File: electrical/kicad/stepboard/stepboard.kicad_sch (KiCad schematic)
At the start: 72 parts, among them J1 Conn_02x03_Odd_Even, J10 Conn_01x04, J4 Conn_01x04, J7 Conn_02x03_Odd_Even, U1 TMC2209, U4 TMC2209

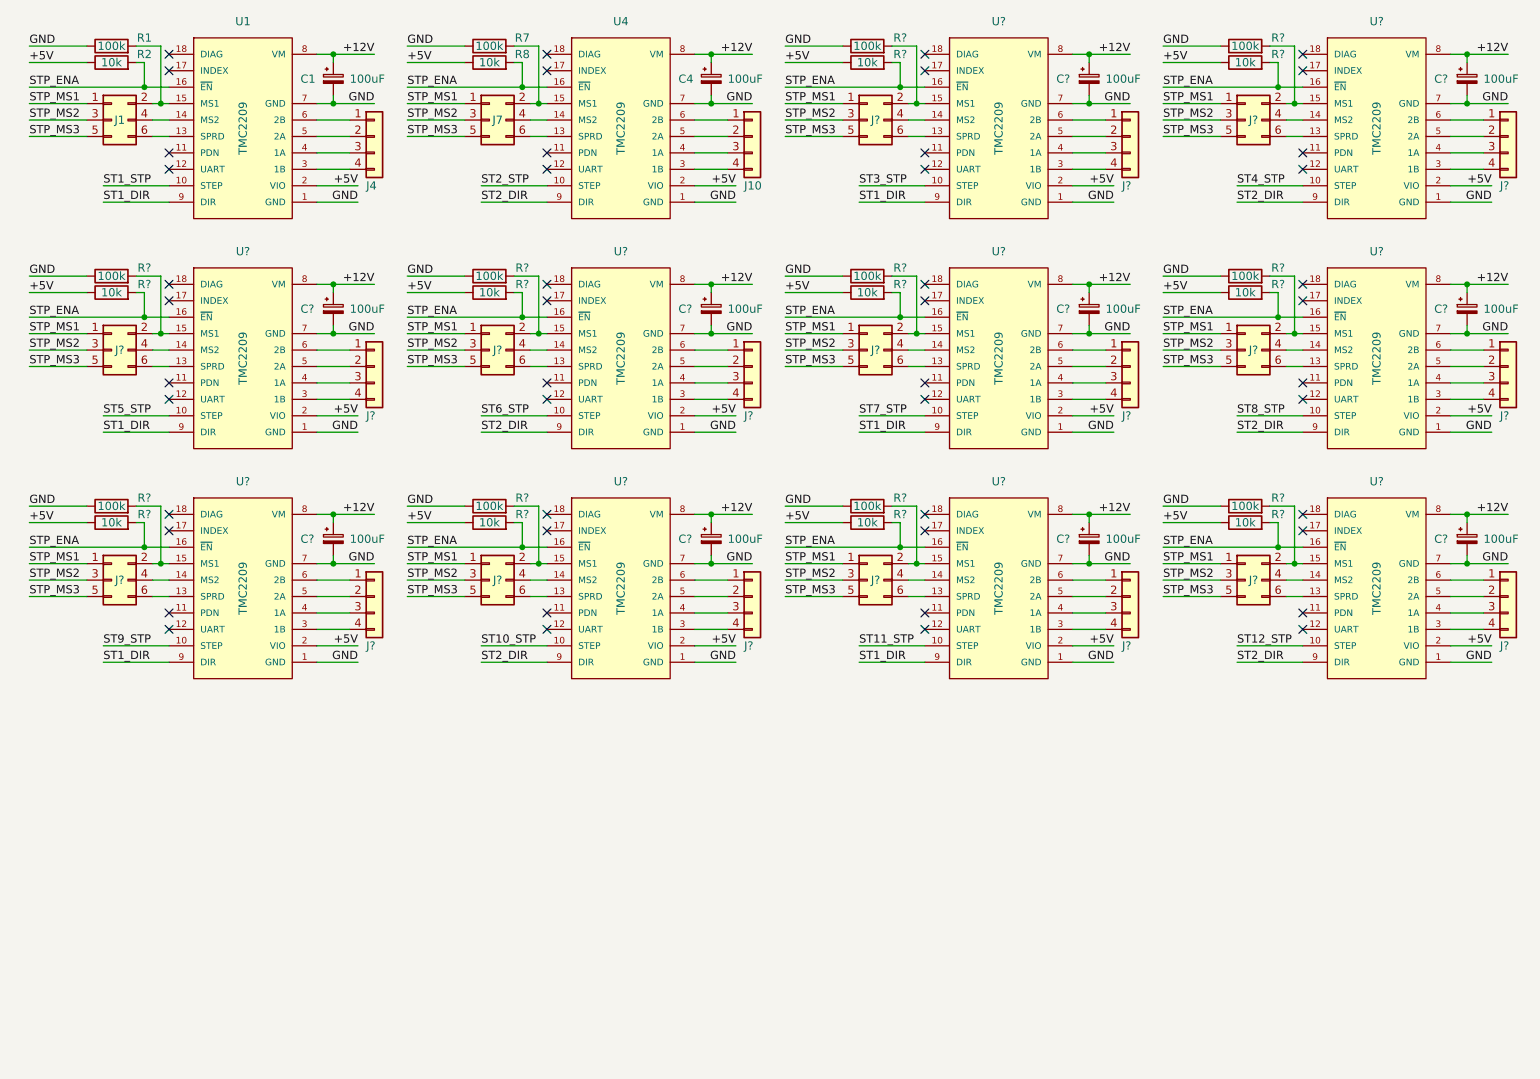
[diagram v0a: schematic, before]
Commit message: update(kicad/step): ERC & DRC Passed
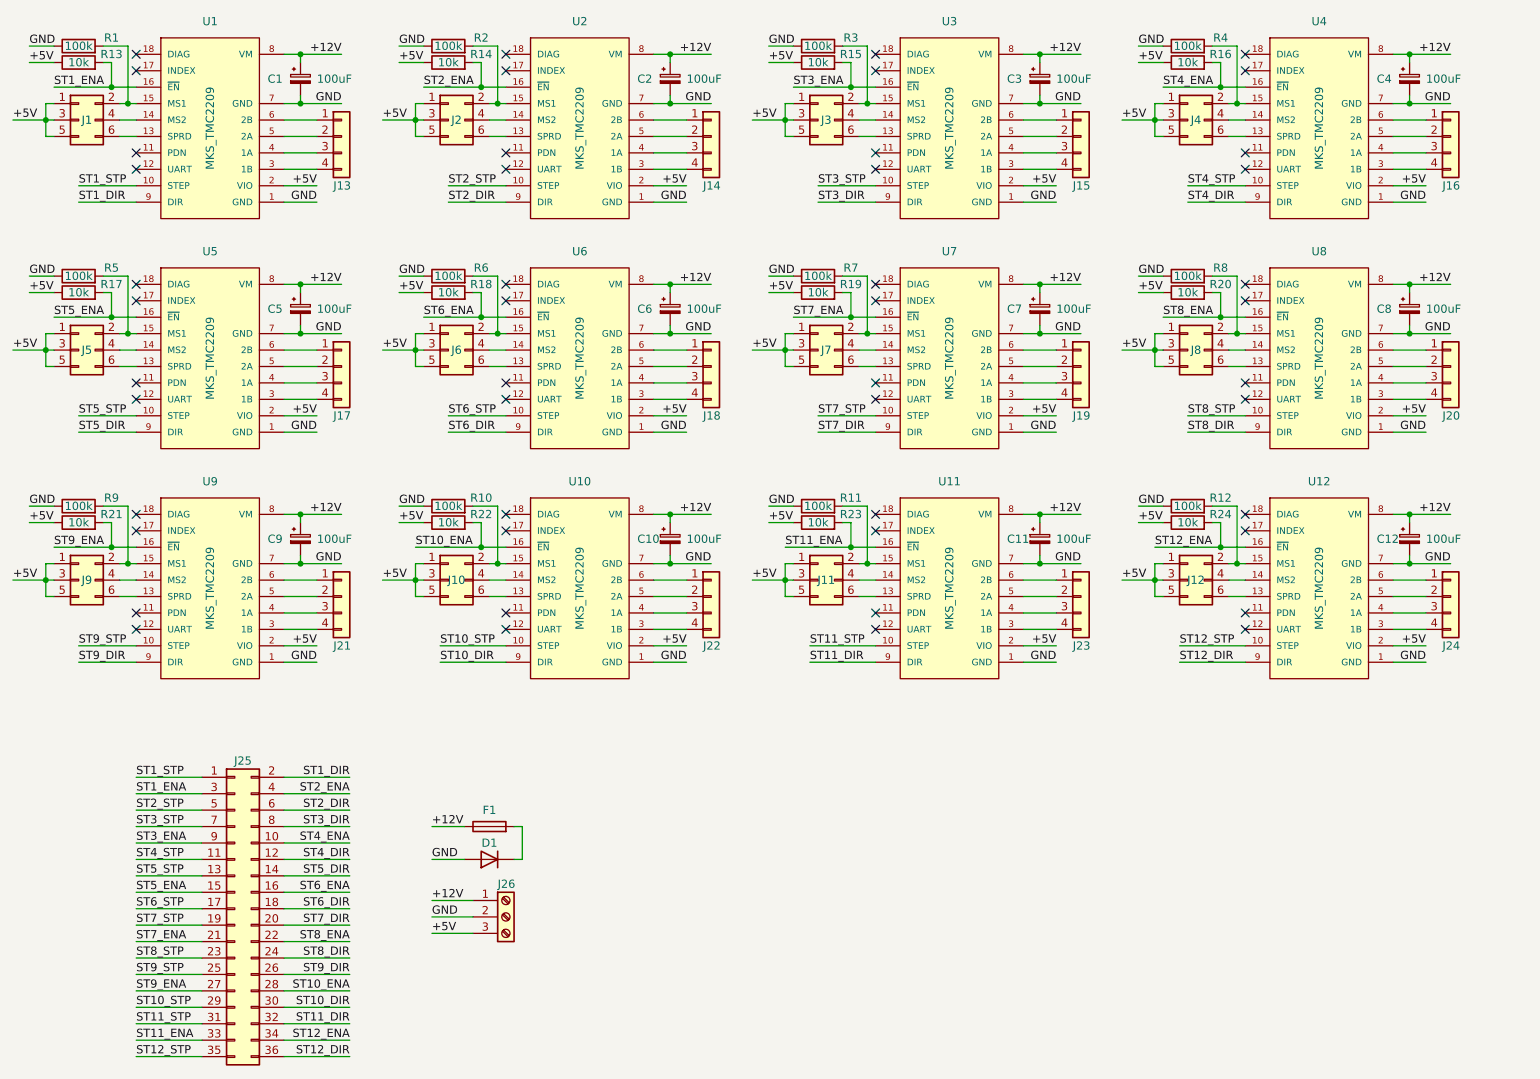
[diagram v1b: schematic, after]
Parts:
- removed C? (x10): 100uF, symbol Device:C_Polarized_Small
- removed J10, J? (x10): Conn_01x04, symbol Connector_Generic:Conn_01x04
- removed J? (x10): Conn_02x03_Odd_Even, symbol Connector_Generic:Conn_02x03_Odd_Even
- removed R? (x10): 10k, symbol Device:R
- removed R? (x10): 100k, symbol Device:R
- removed U? (x10): TMC2209, Motor_Driver:MKS_TMC2209, symbol Motor_Driver:TMC2209_Stepper_Driver
- added C10, C11, C12, C2, C3, C5, C6, C7, C8, C9: 100uF, Capacitors_THT:CP_Radial_D8.0mm_P3.50mm_H12.0mm_Horizontal, symbol Device:C_Polarized_Small
- added D1: D, Diode_THT:D_DO-35_SOD27_P7.62mm_Horizontal, symbol Device:D
- added F1: Fuse, Fuses_THT:Fuse_Tyco-RUEF900, symbol Device:Fuse
- added J10, J11, J12, J2, J3, J4, J5, J6, J8, J9: Conn_02x03_Odd_Even, Connector_PinHeader_2.54mm:PinHeader_2x03_P2.54mm_Vertical, symbol Connector_Generic:Conn_02x03_Odd_Even
- added J14, J15, J16, J17, J18, J19, J20, J21, J22, J23, J24: Conn_01x04, Connector_PinHeader_2.54mm:PinHeader_1x04_P2.54mm_Vertical, symbol Connector_Generic:Conn_01x04
- added J25: Conn_02x18_Odd_Even, Connector_PinHeader_2.54mm:PinHeader_2x18_P2.54mm_Vertical, symbol Connector_Generic:Conn_02x18_Odd_Even
- added J26: Screw_Terminal_01x03, Connector_Phoenix_MSTB:PhoenixContact_MSTBA_2,5_3-G-5,08_1x03_P5.08mm_Horizontal, symbol Connector:Screw_Terminal_01x03
- added R10, R11, R12, R2, R3, R4, R5, R6, R9: 100k, Resistor_THT:R_Axial_DIN0207_L6.3mm_D2.5mm_P7.62mm_Horizontal, symbol Device:R
- added R14, R15, R16, R17, R18, R19, R20, R21, R22, R23, R24: 10k, Resistor_THT:R_Axial_DIN0207_L6.3mm_D2.5mm_P7.62mm_Horizontal, symbol Device:R
- added U10, U11, U12, U2, U3, U5, U6, U7, U8, U9: MKS_TMC2209, Motor_Driver:MKS_TMC2209, symbol Motor_Driver:TMC2209_Stepper_Driver
- C1, C4: footprint (none) -> Capacitors_THT:CP_Radial_D8.0mm_P3.50mm_H12.0mm_Horizontal
- J1, J7: footprint (none) -> Connector_PinHeader_2.54mm:PinHeader_2x03_P2.54mm_Vertical
- J13: renamed from J4; footprint (none) -> Connector_PinHeader_2.54mm:PinHeader_1x04_P2.54mm_Vertical
- R1, R7: footprint (none) -> Resistor_THT:R_Axial_DIN0207_L6.3mm_D2.5mm_P7.62mm_Horizontal
- R13: renamed from R2; footprint (none) -> Resistor_THT:R_Axial_DIN0207_L6.3mm_D2.5mm_P7.62mm_Horizontal
- R8: value 10k -> 100k; footprint (none) -> Resistor_THT:R_Axial_DIN0207_L6.3mm_D2.5mm_P7.62mm_Horizontal
- U1, U4: value TMC2209 -> MKS_TMC2209
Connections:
- net STP_MS1 is gone; now on net +5V: J1.1 (Pin_1), J7.1 (Pin_1)
- net STP_MS2 is gone; now on net +5V: J1.3 (Pin_3), J7.3 (Pin_3)
- net STP_MS3 is gone; now on net +5V: J1.5 (Pin_5), J7.5 (Pin_5)
- net +12V: now also C10.1, C11.1, C12.1, C2.1, C3.1, C5.1, C6.1, C7.1, C8.1, C9.1, F1.1, J26.1 (Pin_1), U10.8 (VM), U11.8 (VM), U12.8 (VM), U2.8 (VM), U3.8 (VM), U5.8 (VM), U6.8 (VM), U7.8 (VM), U8.8 (VM), U9.8 (VM)
- net +5V: now also J10.1 (Pin_1), J10.3 (Pin_3), J10.5 (Pin_5), J11.1 (Pin_1), J11.3 (Pin_3), J11.5 (Pin_5), J12.1 (Pin_1), J12.3 (Pin_3), J12.5 (Pin_5), J2.1 (Pin_1), J2.3 (Pin_3), J2.5 (Pin_5), J26.3 (Pin_3), J3.1 (Pin_1), J3.3 (Pin_3), J3.5 (Pin_5), J4.1 (Pin_1), J4.3 (Pin_3), J4.5 (Pin_5), J5.1 (Pin_1), J5.3 (Pin_3), J5.5 (Pin_5), J6.1 (Pin_1), J6.3 (Pin_3), J6.5 (Pin_5), J8.1 (Pin_1), J8.3 (Pin_3), J8.5 (Pin_5), J9.1 (Pin_1), J9.3 (Pin_3), J9.5 (Pin_5), R14.1, R15.1, R16.1, R17.1, R18.1, R19.1, R20.1, R21.1, R22.1, R23.1, R24.1, U10.2 (VIO), U11.2 (VIO), U12.2 (VIO), U2.2 (VIO), U3.2 (VIO), U5.2 (VIO), U6.2 (VIO), U7.2 (VIO), U8.2 (VIO), U9.2 (VIO); no longer R8.1
- net GND: now also R8.1, C10.2, C11.2, C12.2, C2.2, C3.2, C5.2, C6.2, C7.2, C8.2, C9.2, D1.2 (A), J26.2 (Pin_2), R10.1, R11.1, R12.1, R2.1, R3.1, R4.1, R5.1, R6.1, R9.1, U10.1 (GND), U10.7 (GND), U11.1 (GND), U11.7 (GND), U12.1 (GND), U12.7 (GND), U2.1 (GND), U2.7 (GND), U3.1 (GND), U3.7 (GND), U5.1 (GND), U5.7 (GND), U6.1 (GND), U6.7 (GND), U7.1 (GND), U7.7 (GND), U8.1 (GND), U8.7 (GND), U9.1 (GND), U9.7 (GND)
- net ST10_STP: now also J25.29 (Pin_29), U10.10 (STEP)
- net ST11_STP: now also J25.31 (Pin_31), U11.10 (STEP)
- net ST12_STP: now also J25.35 (Pin_35), U12.10 (STEP)
- net ST1_DIR: now also J25.2 (Pin_2)
- net ST1_STP: now also J25.1 (Pin_1)
- net ST2_DIR: now also J25.6 (Pin_6), U2.9 (DIR); no longer U4.9 (DIR)
- net ST2_STP: now also J25.5 (Pin_5), U2.10 (STEP); no longer U4.10 (STEP)
- net ST3_STP: now also J25.7 (Pin_7), U3.10 (STEP)
- net ST4_STP: now also U4.10 (STEP), J25.11 (Pin_11)
- net ST5_STP: now also J25.13 (Pin_13), U5.10 (STEP)
- net ST6_STP: now also J25.17 (Pin_17), U6.10 (STEP)
- net ST7_STP: now also J25.19 (Pin_19), U7.10 (STEP)
- net ST8_STP: now also J25.23 (Pin_23), U8.10 (STEP)
- net ST9_STP: now also J25.25 (Pin_25), U9.10 (STEP)
- net at J7.2 (Pin_2), R7.2: now also U7.15 (MS1); no longer U4.15 (MS1)
- net at J7.4 (Pin_4): now also U7.14 (MS2); no longer U4.14 (MS2)
- net at J7.6 (Pin_6): now also U7.13 (SPRD); no longer U4.13 (SPRD)
- net at U4.6 (2B): now also J16.1 (Pin_1)
- net at U4.5 (2A): now also J16.2 (Pin_2)
- net at U4.4 (1A): now also J16.3 (Pin_3)
- net at U4.3 (1B): now also J16.4 (Pin_4)
- net STP_ENA renamed ST1_ENA
- net ST1_ENA: now also J25.3 (Pin_3); no longer R8.2, U4.16 (~{EN})
- new net: J11.2 (Pin_2), R11.2, U11.15 (MS1)
- new net: J11.4 (Pin_4), U11.14 (MS2)
- new net: J11.6 (Pin_6), U11.13 (SPRD)
- new net: J8.2 (Pin_2), R8.2, U8.15 (MS1)
- new net: J8.4 (Pin_4), U8.14 (MS2)
- new net: J8.6 (Pin_6), U8.13 (SPRD)
- new net: J14.1 (Pin_1), U2.6 (2B)
- new net: J14.2 (Pin_2), U2.5 (2A)
- new net: J14.3 (Pin_3), U2.4 (1A)
- new net: J14.4 (Pin_4), U2.3 (1B)
- new net: D1.1 (K), F1.2
- new net: J21.1 (Pin_1), U9.6 (2B)
- new net: J21.2 (Pin_2), U9.5 (2A)
- new net: J21.3 (Pin_3), U9.4 (1A)
- new net: J21.4 (Pin_4), U9.3 (1B)
- new net: J5.2 (Pin_2), R5.2, U5.15 (MS1)
- new net: J5.4 (Pin_4), U5.14 (MS2)
- new net: J5.6 (Pin_6), U5.13 (SPRD)
- new net: J9.2 (Pin_2), R9.2, U9.15 (MS1)
- new net: J9.4 (Pin_4), U9.14 (MS2)
- new net: J9.6 (Pin_6), U9.13 (SPRD)
- new net: J19.1 (Pin_1), U7.6 (2B)
- new net: J19.2 (Pin_2), U7.5 (2A)
- new net: J19.3 (Pin_3), U7.4 (1A)
- new net: J19.4 (Pin_4), U7.3 (1B)
- new net: J20.4 (Pin_4), U8.3 (1B)
- new net: J20.3 (Pin_3), U8.4 (1A)
- new net: J20.2 (Pin_2), U8.5 (2A)
- new net: J20.1 (Pin_1), U8.6 (2B)
- new net: J22.1 (Pin_1), U10.6 (2B)
- new net: J22.2 (Pin_2), U10.5 (2A)
- new net: J22.3 (Pin_3), U10.4 (1A)
- new net: J22.4 (Pin_4), U10.3 (1B)
- new net: J12.6 (Pin_6), U12.13 (SPRD)
- new net: J12.4 (Pin_4), U12.14 (MS2)
- new net: J12.2 (Pin_2), R12.2, U12.15 (MS1)
- new net: J24.4 (Pin_4), U12.3 (1B)
- new net: J24.3 (Pin_3), U12.4 (1A)
- new net: J24.2 (Pin_2), U12.5 (2A)
- new net: J24.1 (Pin_1), U12.6 (2B)
- new net: J2.6 (Pin_6), U2.13 (SPRD)
- new net: J2.4 (Pin_4), U2.14 (MS2)
- new net: J2.2 (Pin_2), R2.2, U2.15 (MS1)
- new net: J3.2 (Pin_2), R3.2, U3.15 (MS1)
- new net: J3.4 (Pin_4), U3.14 (MS2)
- new net: J3.6 (Pin_6), U3.13 (SPRD)
- new net: J6.6 (Pin_6), U6.13 (SPRD)
- new net: J6.4 (Pin_4), U6.14 (MS2)
- new net: J6.2 (Pin_2), R6.2, U6.15 (MS1)
- new net: J18.4 (Pin_4), U6.3 (1B)
- new net: J18.3 (Pin_3), U6.4 (1A)
- new net: J18.2 (Pin_2), U6.5 (2A)
- new net: J18.1 (Pin_1), U6.6 (2B)
- new net: J10.2 (Pin_2), R10.2, U10.15 (MS1)
- new net: J10.4 (Pin_4), U10.14 (MS2)
- new net: J10.6 (Pin_6), U10.13 (SPRD)
- new net: J23.4 (Pin_4), U11.3 (1B)
- new net: J23.3 (Pin_3), U11.4 (1A)
- new net: J23.2 (Pin_2), U11.5 (2A)
- new net: J23.1 (Pin_1), U11.6 (2B)
- new net: J4.2 (Pin_2), R4.2, U4.15 (MS1)
- new net: J4.4 (Pin_4), U4.14 (MS2)
- new net: J4.6 (Pin_6), U4.13 (SPRD)
- new net: J17.4 (Pin_4), U5.3 (1B)
- new net: J17.3 (Pin_3), U5.4 (1A)
- new net: J17.2 (Pin_2), U5.5 (2A)
- new net: J17.1 (Pin_1), U5.6 (2B)
- new net: J15.4 (Pin_4), U3.3 (1B)
- new net: J15.3 (Pin_3), U3.4 (1A)
- new net: J15.2 (Pin_2), U3.5 (2A)
- new net: J15.1 (Pin_1), U3.6 (2B)
- new net ST10_DIR: J25.30 (Pin_30), U10.9 (DIR)
- new net ST10_ENA: J25.28 (Pin_28), R22.2, U10.16 (~{EN})
- new net ST11_DIR: J25.32 (Pin_32), U11.9 (DIR)
- new net ST11_ENA: J25.33 (Pin_33), R23.2, U11.16 (~{EN})
- new net ST12_DIR: J25.36 (Pin_36), U12.9 (DIR)
- new net ST12_ENA: J25.34 (Pin_34), R24.2, U12.16 (~{EN})
- new net ST2_ENA: J25.4 (Pin_4), R14.2, U2.16 (~{EN})
- new net ST3_DIR: J25.8 (Pin_8), U3.9 (DIR)
- new net ST3_ENA: J25.9 (Pin_9), R15.2, U3.16 (~{EN})
- new net ST4_DIR: J25.12 (Pin_12), U4.9 (DIR)
- new net ST4_ENA: J25.10 (Pin_10), R16.2, U4.16 (~{EN})
- new net ST5_DIR: J25.14 (Pin_14), U5.9 (DIR)
- new net ST5_ENA: J25.15 (Pin_15), R17.2, U5.16 (~{EN})
- new net ST6_DIR: J25.18 (Pin_18), U6.9 (DIR)
- new net ST6_ENA: J25.16 (Pin_16), R18.2, U6.16 (~{EN})
- new net ST7_DIR: J25.20 (Pin_20), U7.9 (DIR)
- new net ST7_ENA: J25.21 (Pin_21), R19.2, U7.16 (~{EN})
- new net ST8_DIR: J25.24 (Pin_24), U8.9 (DIR)
- new net ST8_ENA: J25.22 (Pin_22), R20.2, U8.16 (~{EN})
- new net ST9_DIR: J25.26 (Pin_26), U9.9 (DIR)
- new net ST9_ENA: J25.27 (Pin_27), R21.2, U9.16 (~{EN})
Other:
- moved on the sheet: C1, J13, R1, R13, U1
